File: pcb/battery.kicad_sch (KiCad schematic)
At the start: 10 parts, among them U8 AMS1117-3.3, U9 TP4056-42-ESOP8

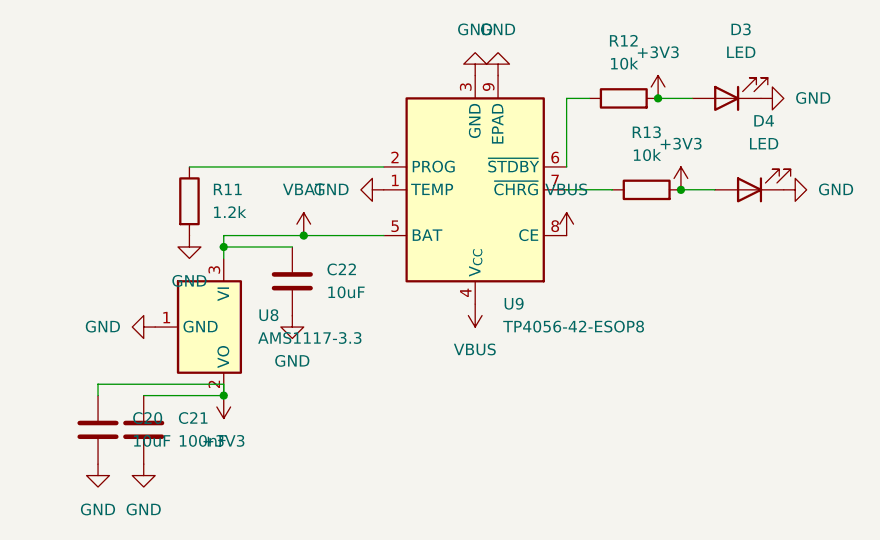
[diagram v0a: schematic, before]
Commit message: Add files via upload
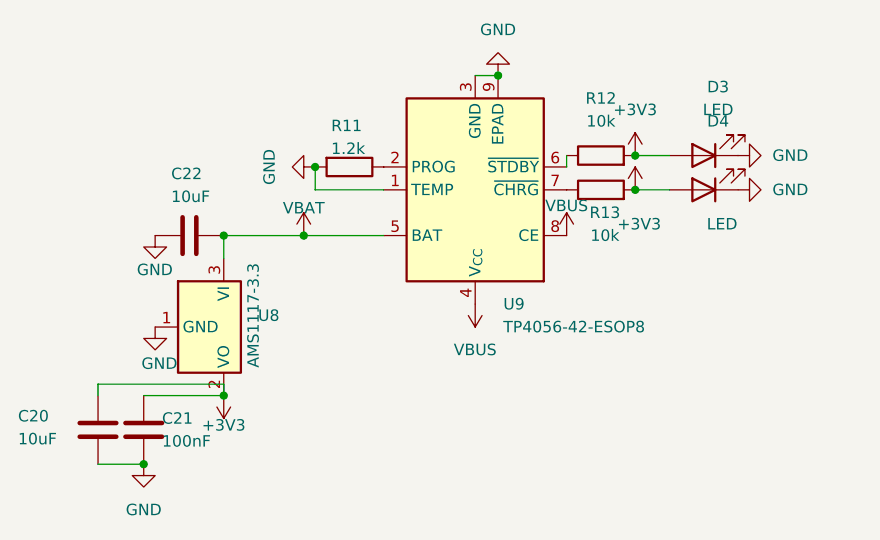
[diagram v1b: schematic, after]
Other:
- moved on the sheet: C22, D3, D4, R11, R12, R13
